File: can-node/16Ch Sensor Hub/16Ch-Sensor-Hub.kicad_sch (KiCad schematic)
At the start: 58 parts, among them J1 Conn_ARM_JTAG_SWD_10, J2 Conn_01x04_Pin, J3 Conn_01x02, J4 Conn_02x06_Top_Bottom, J5 Conn_02x06_Top_Bottom, J6 Conn_02x06_Top_Bottom, J7 Conn_02x06_Top_Bottom, Q2 DMP510DL-7, SW1 RESET, U1 TCAN3404-Q1, U2 STM32F105RBTx, U20 ISM330DHCX, U21 MCP9800Ax-xOT, U3 AP7375Q-33SF, Y1 ECS-250-10-47Q-CES-TR

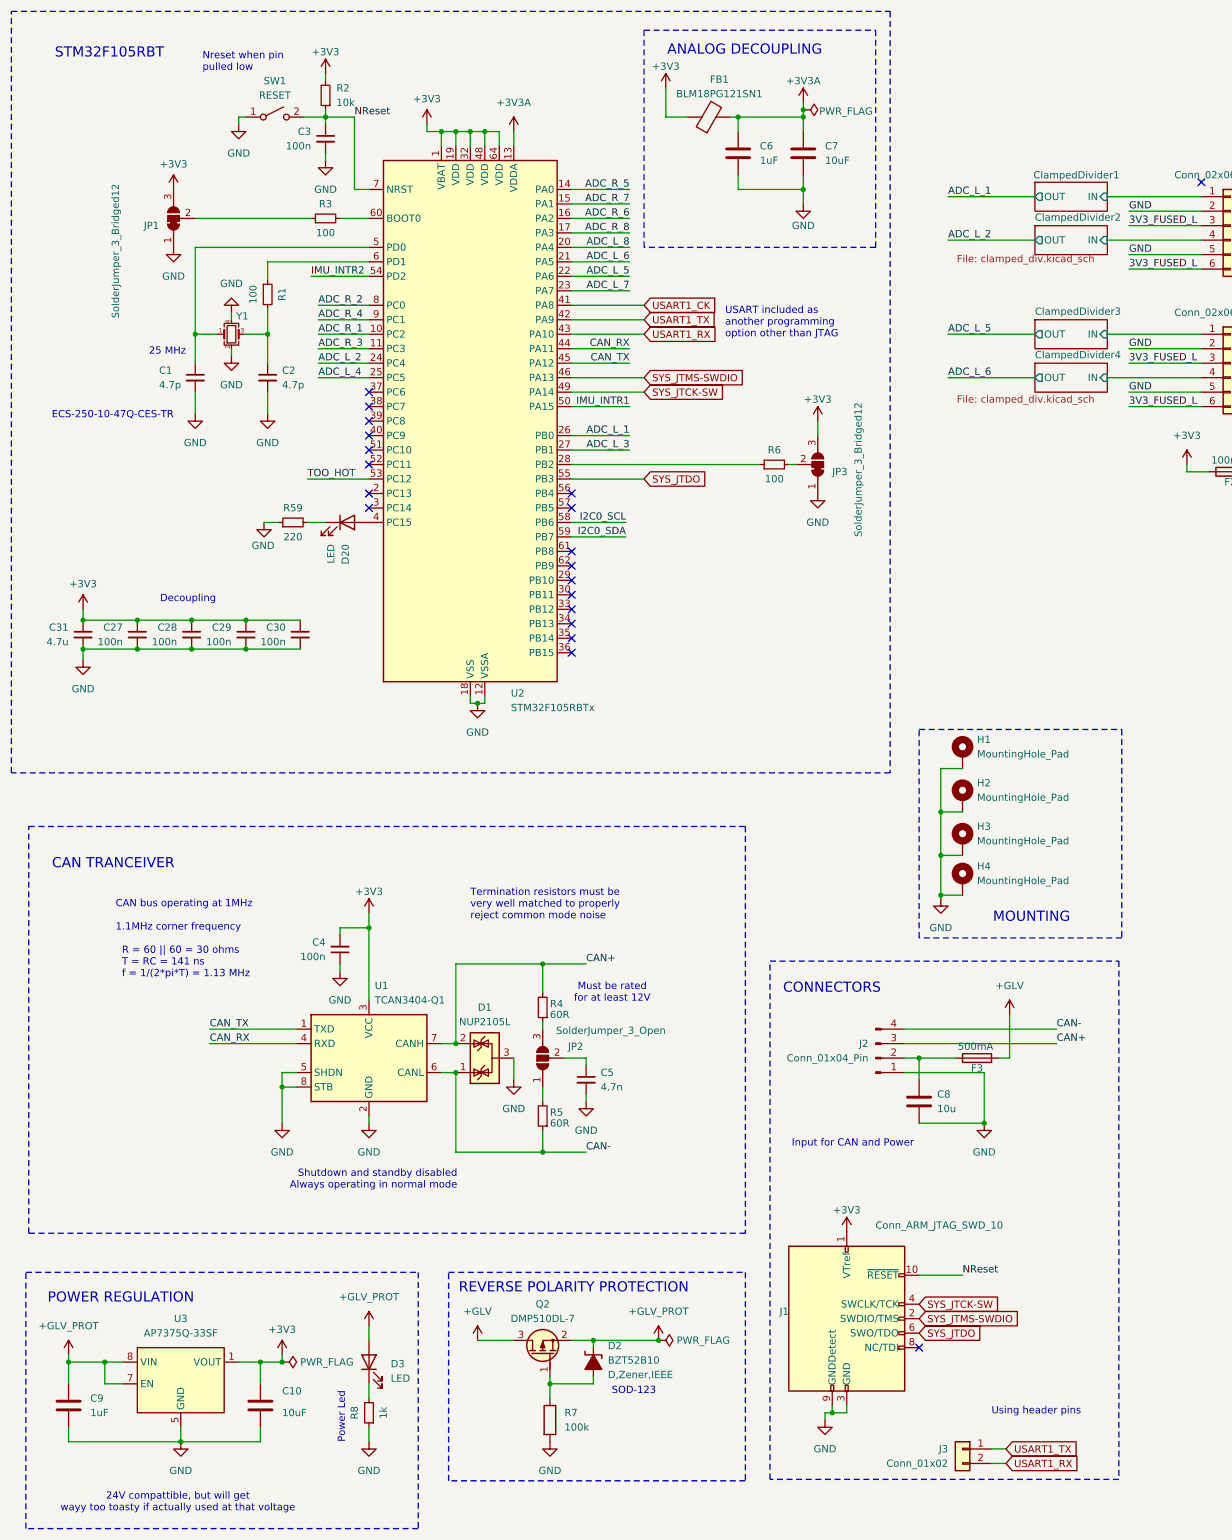
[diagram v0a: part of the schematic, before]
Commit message: 1.0.0 Release
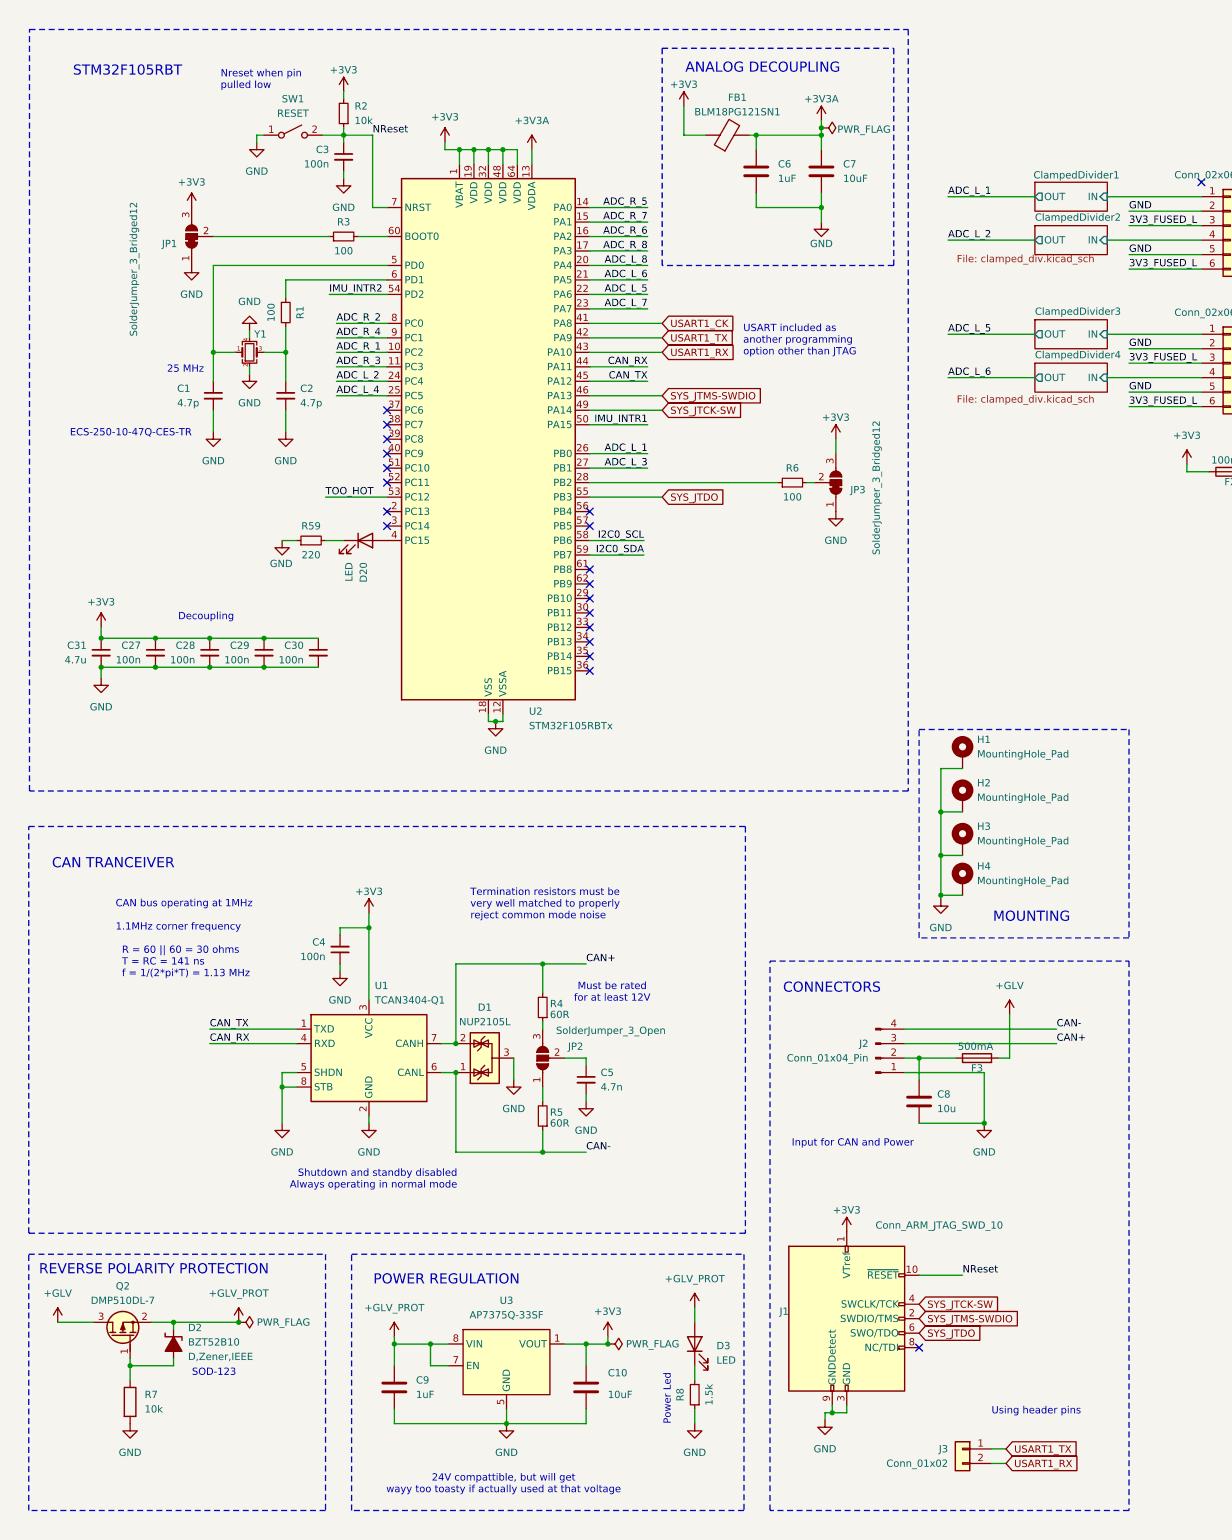
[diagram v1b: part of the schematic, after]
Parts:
- R7: value 100k -> 10k
- R8: value 1k -> 1.5k
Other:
- moved on the sheet: C1, C10, C2, C27, C28, C29, C3, C30, C31, C6, C7, C9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
